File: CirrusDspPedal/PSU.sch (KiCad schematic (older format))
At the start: 6 parts, among them J4 Barrel_Jack_Switch, J7 Conn_01x01, U5 MCP1703A-1202_SOT223

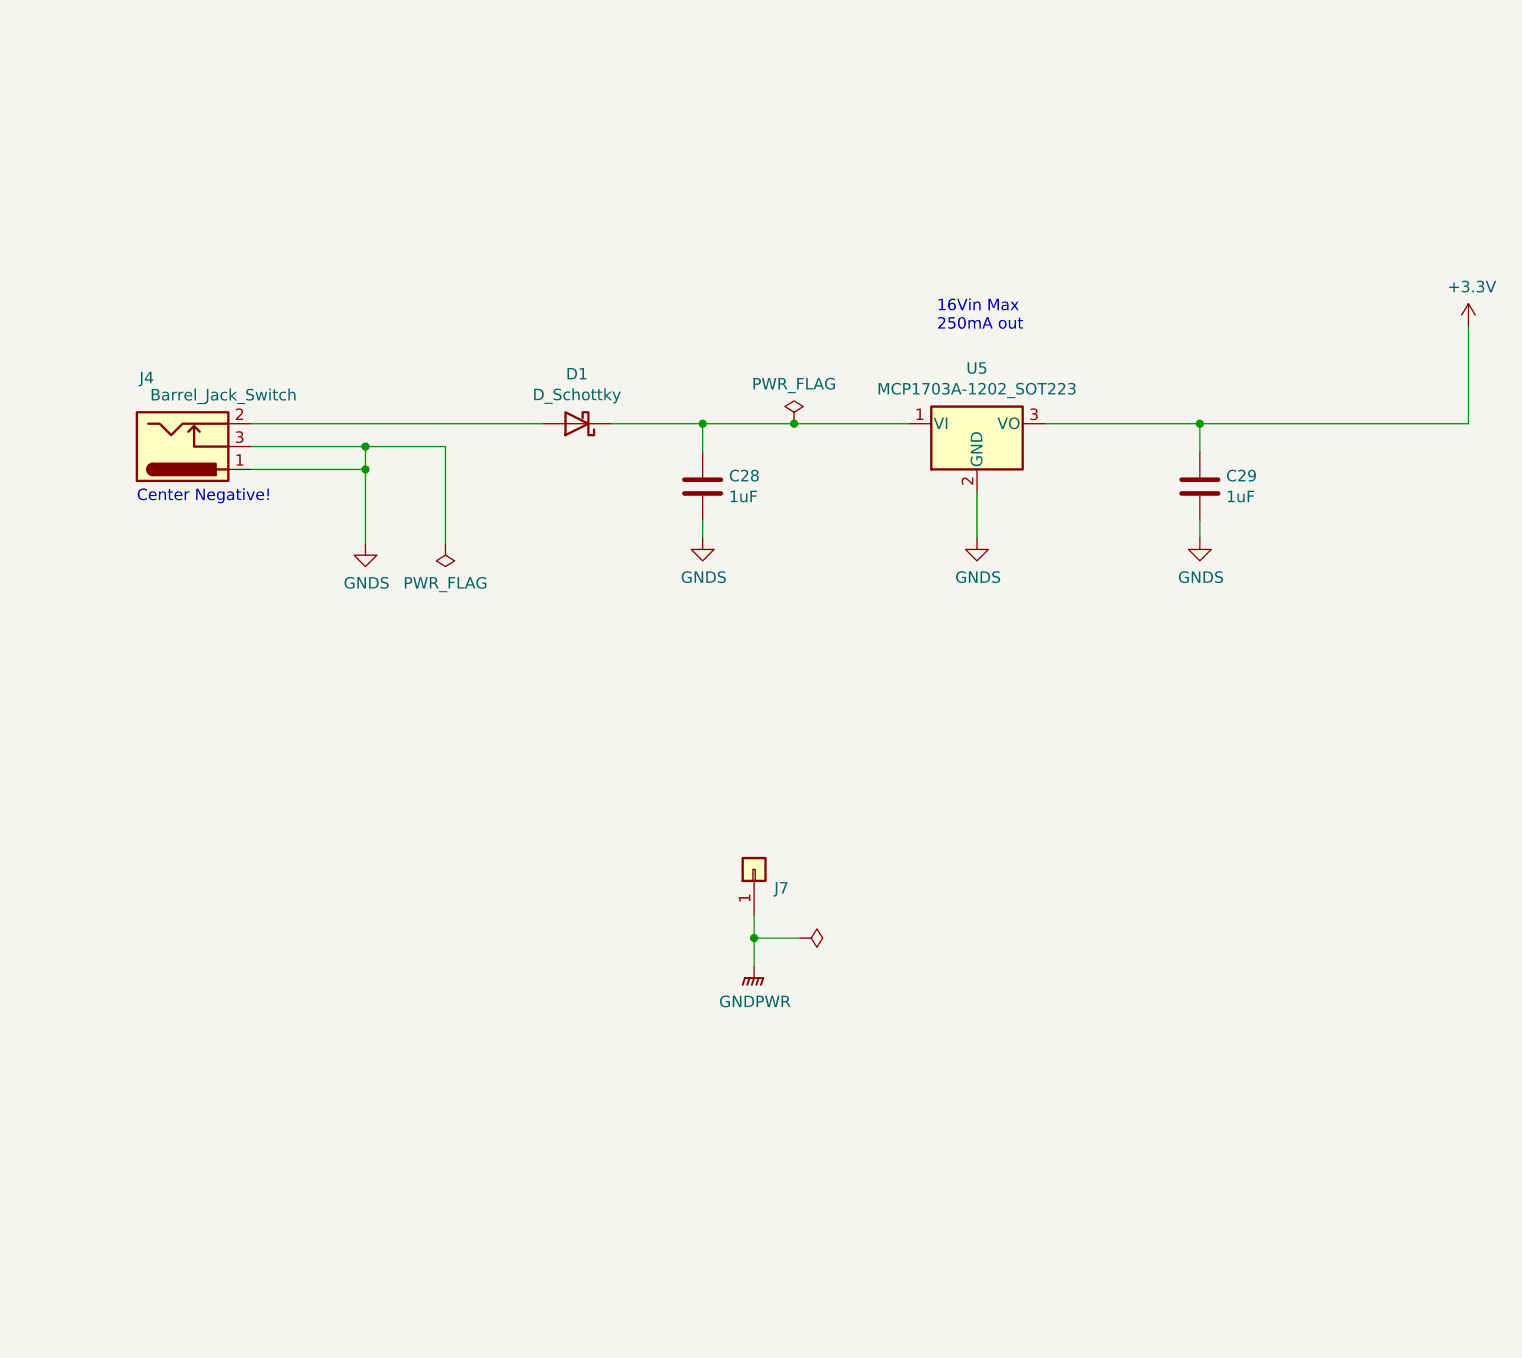
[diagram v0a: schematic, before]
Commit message: finished revb layout
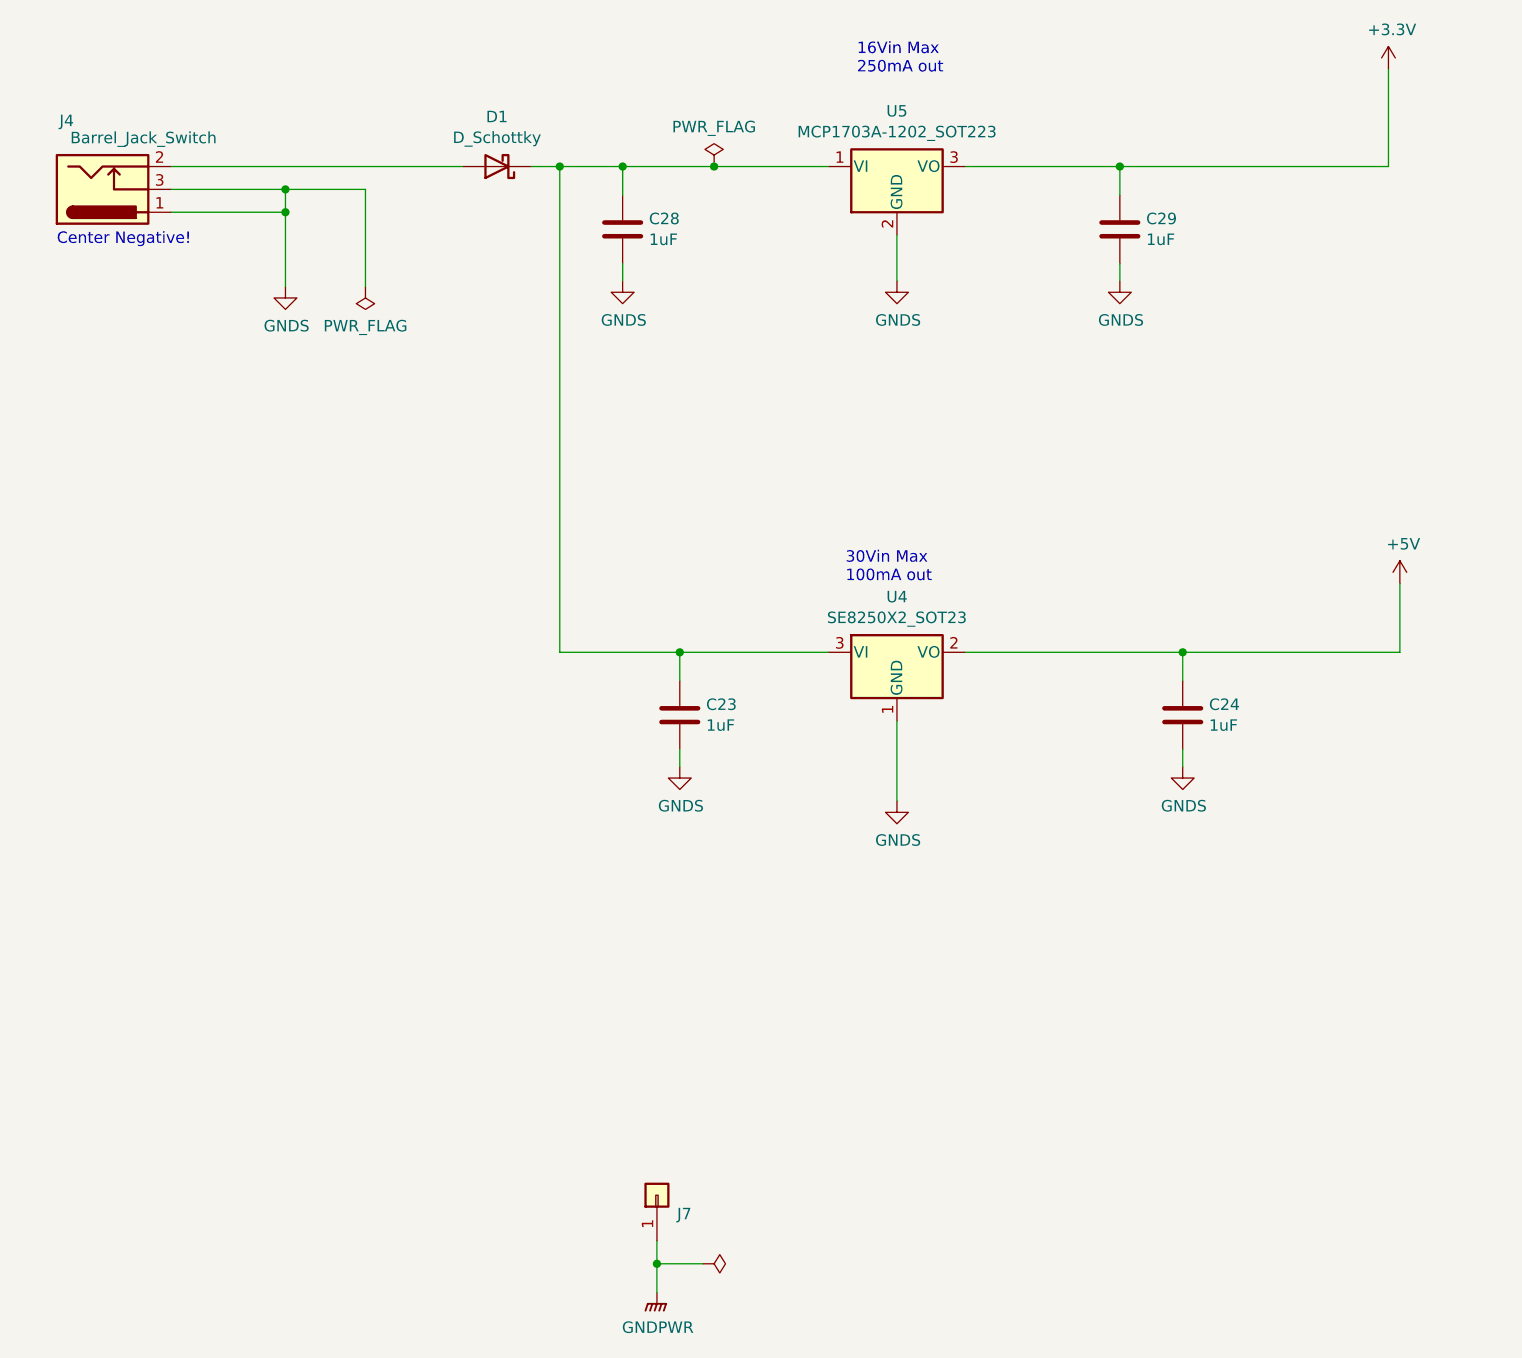
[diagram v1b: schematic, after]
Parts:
- added C23, C24: 1uF, Capacitor_SMD:C_1206_3216Metric_Pad1.42x1.75mm_HandSolder, symbol Device:C
- added U4: SE8250X2_SOT23, Package_TO_SOT_SMD:SOT-23, symbol Regulator_Linear:MCP1700-5002E_SOT23
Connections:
- net GNDS: now also C23.2, C24.2, U4.1 (GND)
- net at C28.1, D1.1 (K), U5.1 (VI): now also C23.1, U4.3 (VI)
- new net +5V: C24.1, U4.2 (VO)
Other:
- note added: "30Vin Max\n100mA out"
- moved on the sheet: C28, C29, D1, J4, J7, U5
